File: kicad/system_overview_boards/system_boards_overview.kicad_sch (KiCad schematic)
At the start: 0 parts

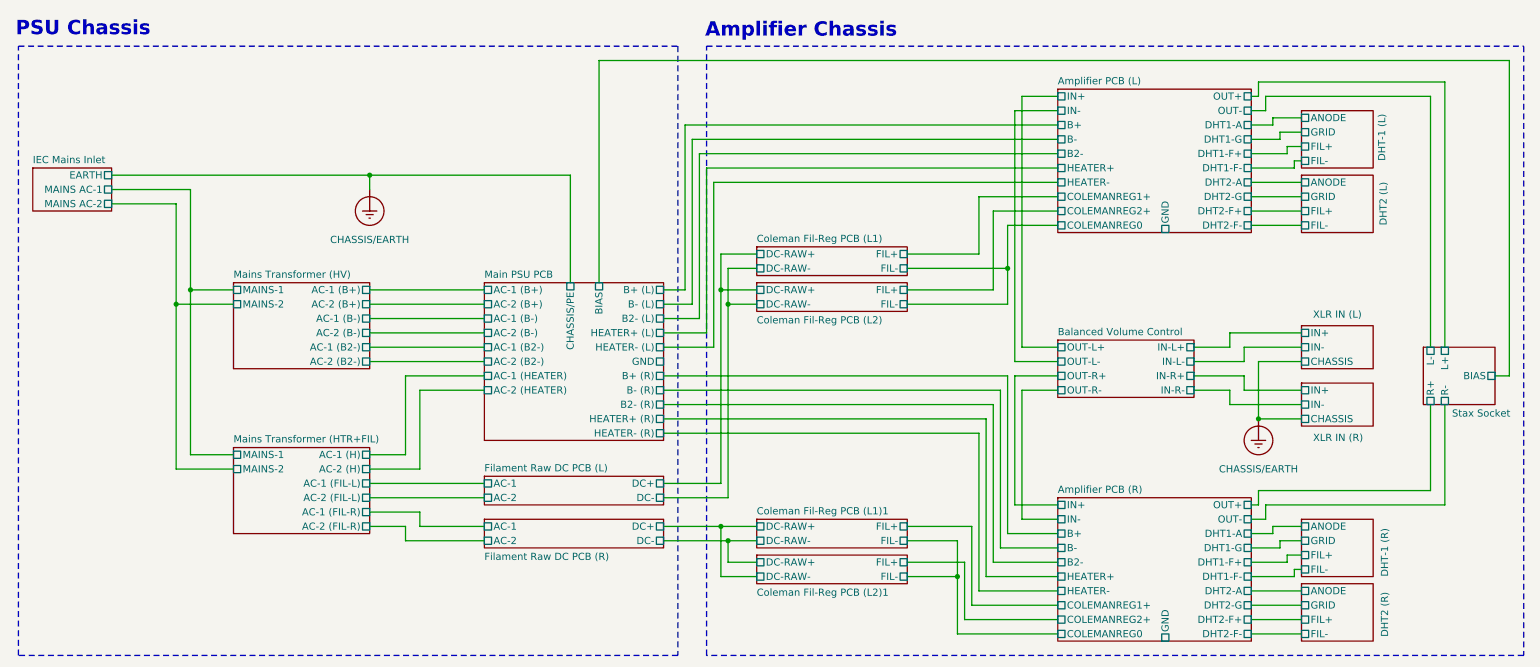
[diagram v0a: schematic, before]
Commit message: system overview
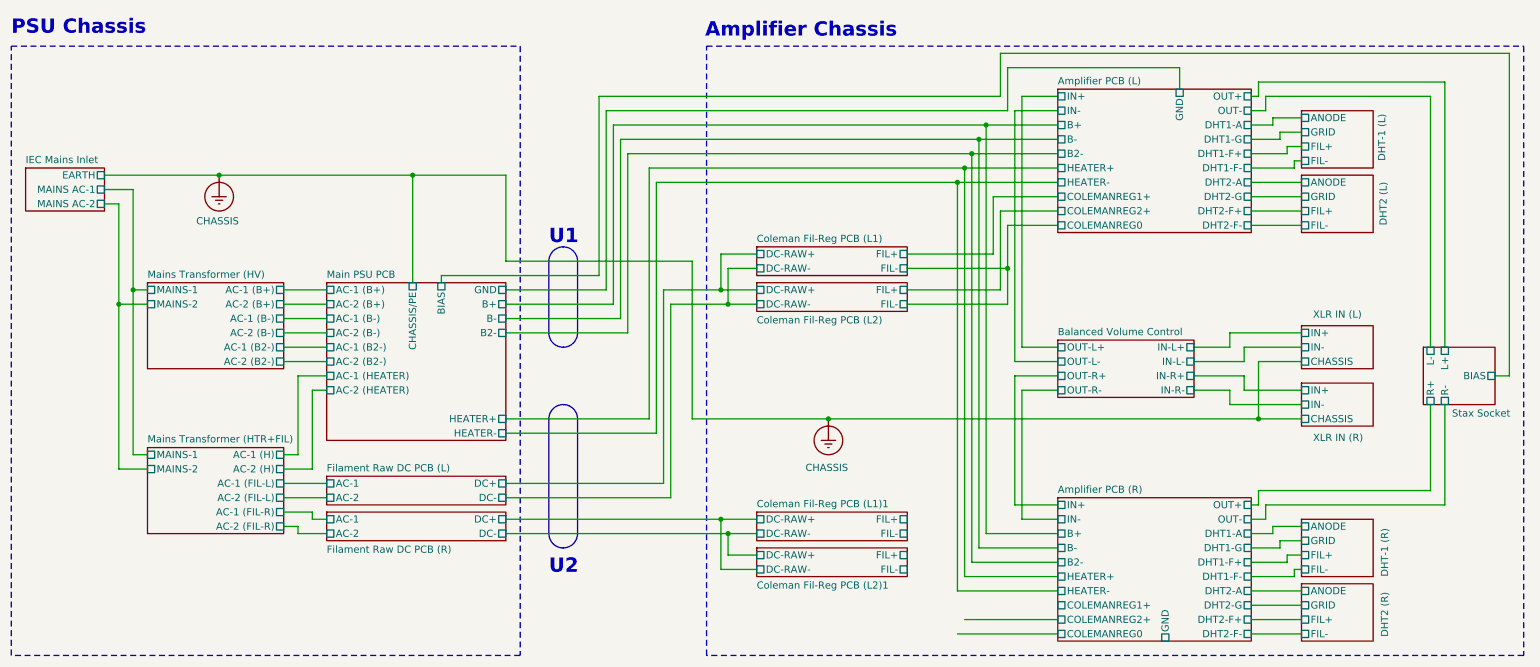
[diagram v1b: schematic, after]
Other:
- sheet Main PSU PCB ports: added B+, B-, B2-, HEATER+, HEATER-; removed B+ (L), B+ (R), B- (L), B- (R), B2- (L), B2- (R), HEATER+ (L), HEATER+ (R), HEATER- (L), HEATER- (R)
- note added: "U1"
- note added: "U2"
